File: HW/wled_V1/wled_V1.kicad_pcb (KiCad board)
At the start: 2 copper layers, 32 parts, among them U3 TXS0102DCT

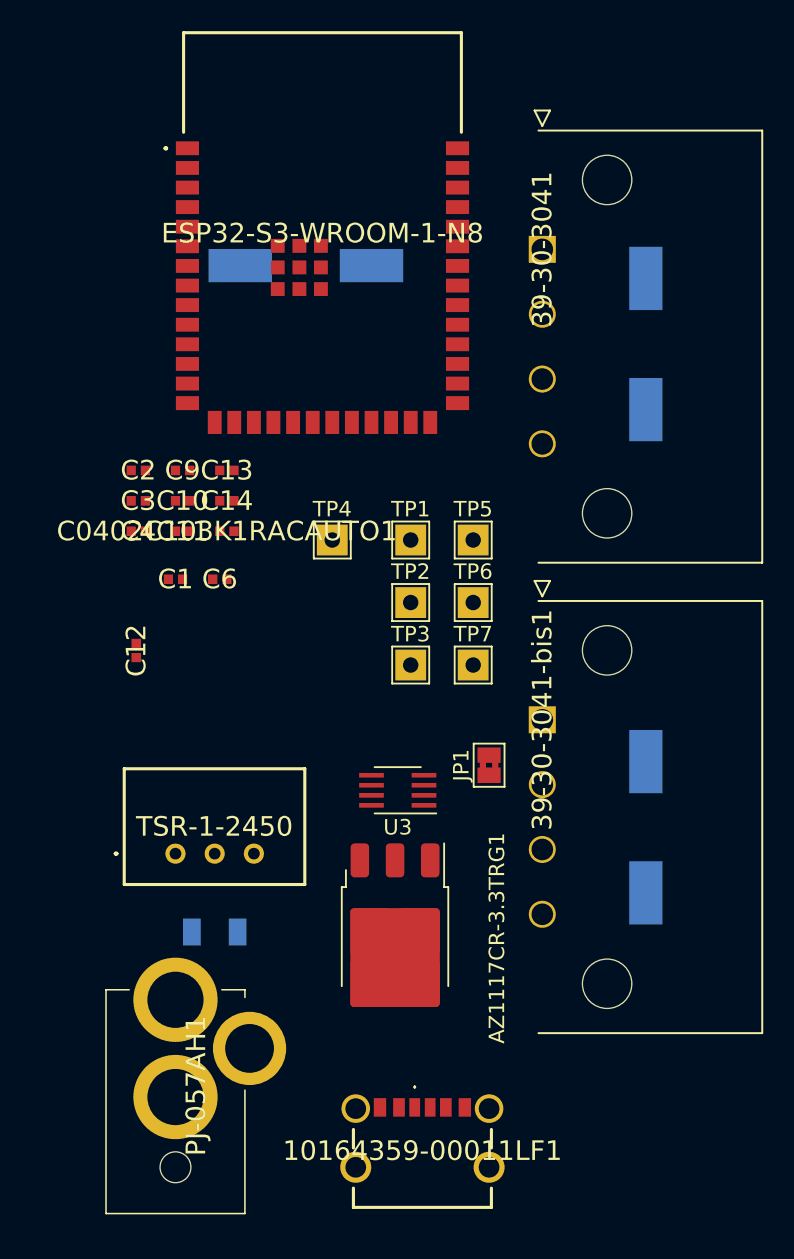
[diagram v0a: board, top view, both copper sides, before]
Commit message: routing
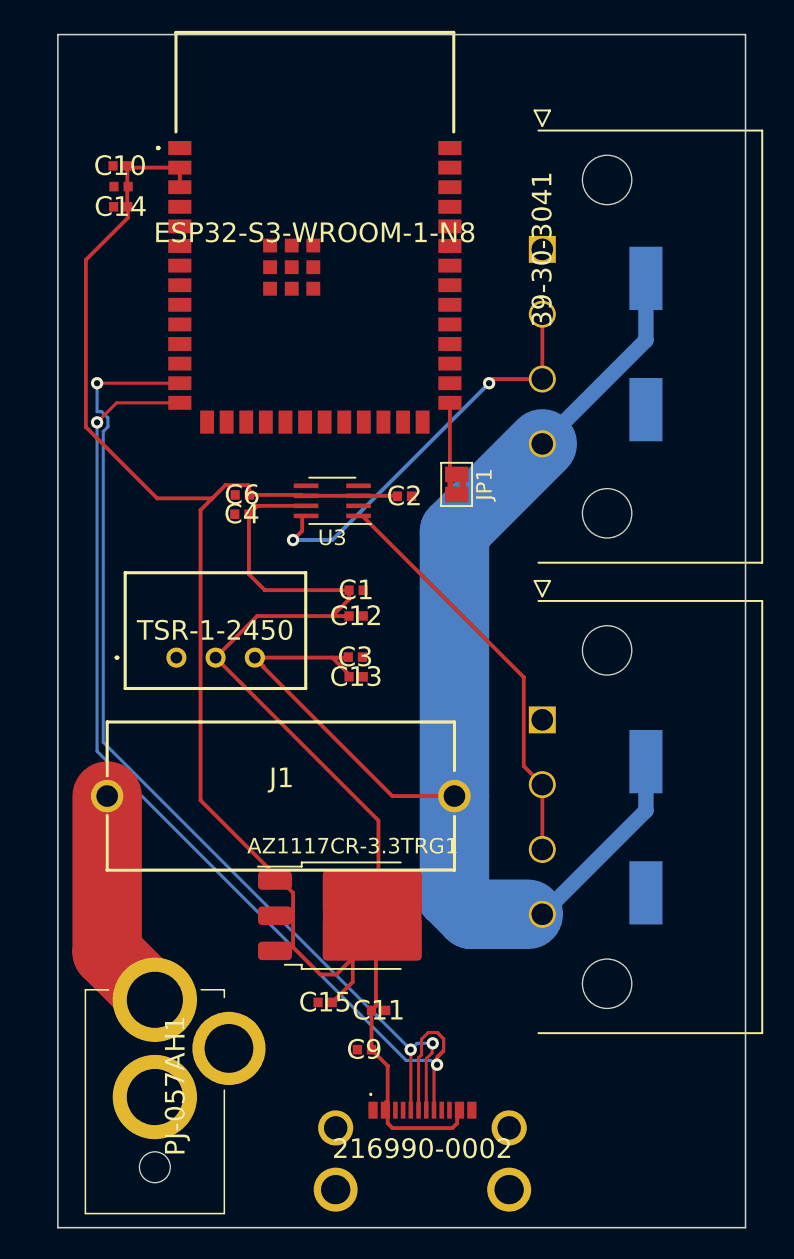
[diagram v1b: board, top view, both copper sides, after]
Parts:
- removed 0440007.WRA1: Fuse, SamacSys_Parts:FUSC3216X85N
- removed TP1, TP2, TP3, TP4, TP5, TP6, TP7: TestPoint, TestPoint:TestPoint_THTPad_2.0x2.0mm_Drill1.0mm
- added J1: 0031.8201, SamacSys_Parts:0031.8201, F.Cu at (118.6, 118.2)
- 216990-0002: renamed from 10164359-00011LF1; footprint SamacSys_Parts:1016435900011LF -> SamacSys_Parts:2169900002
- C15: footprint SamacSys_Parts:CAPAE1030X1030N -> SamacSys_Parts:CAPC1005X55N; moved to F.Cu
- moved C15 47.8 mm to (121.5, 131.6)
- moved C9 39.3 mm to (124.0, 134.6), turned to 180 degrees
- moved C11 33.5 mm to (124.9, 132.1)
- moved C0402C103K1RACAUTO1 23.4 mm to (108.2, 78.7), turned to 180 degrees
- moved C10 22.1 mm to (108.2, 77.4), turned to 180 degrees
- moved C14 20.3 mm to (108.2, 80.0), turned to 180 degrees
- moved U3 19.2 mm to (121.9, 99.1)
- moved JP1 18.3 mm to (130.0, 98.0), turned to -90 degrees
- moved C3 17.3 mm to (123.4, 109.2)
- moved C2 17.3 mm to (126.6, 98.8)
- moved C13 15.8 mm to (123.5, 110.5)
- moved C12 14.4 mm to (123.5, 106.5), turned to 0 degrees
- moved TSR-1-2450 12.7 mm to (111.8, 109.2)
- moved C1 11.7 mm to (123.5, 104.8)
- moved C4 6.80 mm to (116.1, 99.9), turned to 180 degrees
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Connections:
- 216990-0002 pad MH1: (no net) -> unconnected-(216990-0002-PadMH1)
- 216990-0002 pad MH2: (no net) -> unconnected-(216990-0002-PadMH2)
- 216990-0002 pad MH3: (no net) -> unconnected-(216990-0002-PadMH3)
- 216990-0002 pad MH4: (no net) -> unconnected-(216990-0002-PadMH4)
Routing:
- net +12V: track 0.00 -> 87.8 mm
- net +3.3V: track 0.00 -> 86.5 mm
- net D+: track 0.00 -> 71.4 mm, vias 0 -> 2
- net D-: track 0.00 -> 68.4 mm, vias 0 -> 3
- net +5V: track 0.00 -> 68.0 mm
- net Net-(39-30-3041-Pin_2): track 0.00 -> 26.5 mm, vias 0 -> 2
- net Net-(39-30-3041-bis1-Pin_2): track 0.00 -> 26.4 mm
- net Net-(J1-Pad1): track 0.00 -> 16.1 mm
- net Net-(ESP32-S3-WROOM-1-N8-GPIO0/BOOT): track 0.00 -> 4.64 mm
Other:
- board outline added: 44.6 x 77.3 mm
